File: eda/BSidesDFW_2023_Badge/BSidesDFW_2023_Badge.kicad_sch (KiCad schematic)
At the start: 5 parts

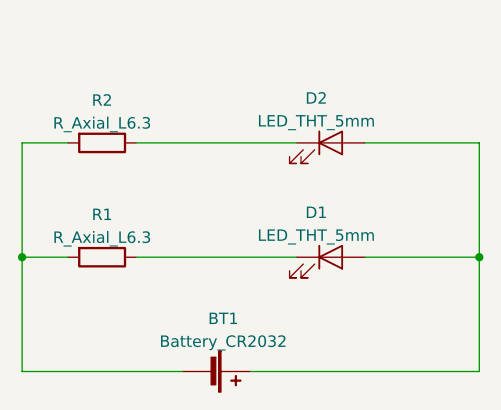
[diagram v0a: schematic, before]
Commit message: document and website updates
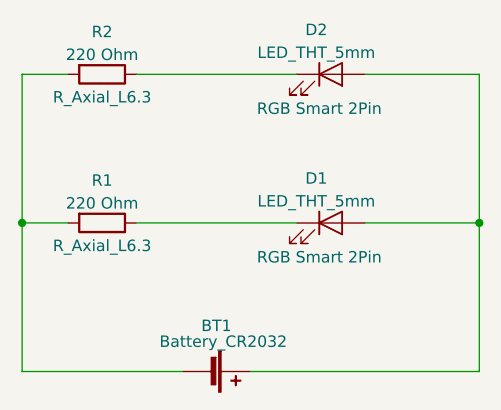
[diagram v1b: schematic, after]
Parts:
- D1, D2: Pkg (none) -> RGB Smart 2Pin
- R1, R2: value R_Axial_L6.3 -> 220 Ohm; Pkg (none) -> R_Axial_L6.3
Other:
- moved on the sheet: D1, D2, R1, R2
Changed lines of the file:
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@@
     (company "Crafted by @alt_bier a.k.a. Richard Gowen")
   )
-  (junction (at 114.3 114.3) (diameter 0) (color 0 0 0 0)
+  (junction (at 165.1 110.49) (diameter 0) (color 0 0 0 0)
   )
-  (junction (at 165.1 114.3) (diameter 0) (color 0 0 0 0)
+  (junction (at 114.3 110.49) (diameter 0) (color 0 0 0 0)
   )
-  (wire (pts (xy 114.3 101.6) (xy 114.3 114.3))
+  (wire (pts (xy 114.3 93.98) (xy 114.3 110.49))
     (stroke (width 0) (type default) (color 0 0 0 0))
   )
-  (wire (pts (xy 165.1 101.6) (xy 152.4 101.6))
+  (wire (pts (xy 165.1 93.98) (xy 152.4 93.98))
     (stroke (width 0) (type default) (color 0 0 0 0))
   )
-  (wire (pts (xy 119.38 101.6) (xy 114.3 101.6))
+  (wire (pts (xy 165.1 110.49) (xy 165.1 93.98))
     (stroke (width 0) (type default) (color 0 0 0 0))
   )
-  (wire (pts (xy 144.78 114.3) (xy 127 114.3))
+  (wire (pts (xy 165.1 110.49) (xy 165.1 127))
     (stroke (width 0) (type default) (color 0 0 0 0))
   )
-  (wire (pts (xy 114.3 114.3) (xy 114.3 127))
+  (wire (pts (xy 119.38 93.98) (xy 114.3 93.98))
+    (stroke (width 0) (type default) (color 0 0 0 0))
+  )
+  (wire (pts (xy 144.78 110.49) (xy 127 110.49))
     (stroke (width 0) (type default) (color 0 0 0 0))
   )
@@
     (stroke (width 0) (type default) (color 0 0 0 0))
   )
-  (wire (pts (xy 144.78 101.6) (xy 127 101.6))
+  (wire (pts (xy 144.78 93.98) (xy 127 93.98))
     (stroke (width 0) (type default) (color 0 0 0 0))
   )
-  (wire (pts (xy 165.1 127) (xy 165.1 114.3))
+  (wire (pts (xy 114.3 110.49) (xy 114.3 127))
     (stroke (width 0) (type default) (color 0 0 0 0))
   )
-  (wire (pts (xy 165.1 114.3) (xy 152.4 114.3))
+  (wire (pts (xy 165.1 110.49) (xy 152.4 110.49))
     (stroke (width 0) (type default) (color 0 0 0 0))
   )
-  (wire (pts (xy 119.38 114.3) (xy 114.3 114.3))
-    (stroke (width 0) (type default) (color 0 0 0 0))
-  )
-  (wire (pts (xy 165.1 114.3) (xy 165.1 101.6))
+  (wire (pts (xy 119.38 110.49) (xy 114.3 110.49))
     (stroke (width 0) (type default) (color 0 0 0 0))
   )
@@
     (stroke (width 0) (type default) (color 0 0 0 0))
   )
-  (symbol (lib_id "0_local:LED_THT_5mm") (at 148.59 114.3 0) (unit 1)
-    (in_bom yes) (on_board yes) (fields_autoplaced)
-    (property "Reference" "D1" (id 0) (at 146.9898 109.3556 0))
-    (property "Value" "LED_THT_5mm" (id 1) (at 146.9898 111.8925 0))
-    (property "Footprint" "0_local:LED_D5.0mm-2" (id 2) (at 148.59 120.65 0)
+  (symbol (lib_id "0_local:LED_THT_5mm") (at 148.59 110.49 0) (unit 1)
+    (in_bom yes) (on_board yes)
+    (property "Reference" "D1" (id 0) (at 146.9898 105.5456 0))
+    (property "Value" "LED_THT_5mm" (id 1) (at 146.9898 108.0825 0))
+    (property "Footprint" "0_local:LED_D5.0mm-2" (id 2) (at 148.59 116.84 0)
       (effects (font (size 1.27 1.27)) hide)
     )
-    (property "Datasheet" "~" (id 3) (at 148.59 114.3 0)
+    (property "Datasheet" "~" (id 3) (at 148.59 110.49 0)
       (effects (font (size 1.27 1.27)) hide)
     )
+    (property "Pkg" "RGB Smart 2Pin" (id 4) (at 147.32 114.3 0))
     (pin "1")
     (pin "2")
   )
-  (symbol (lib_id "0_local:LED_THT_5mm") (at 148.59 101.6 0) (unit 1)
-    (in_bom yes) (on_board yes) (fields_autoplaced)
-    (property "Reference" "D2" (id 0) (at 146.9898 96.6556 0))
-    (property "Value" "LED_THT_5mm" (id 1) (at 146.9898 99.1925 0))
-    (property "Footprint" "0_local:LED_D5.0mm-2" (id 2) (at 148.59 107.95 0)
+  (symbol (lib_id "0_local:LED_THT_5mm") (at 148.59 93.98 0) (unit 1)
+    (in_bom yes) (on_board yes)
+    (property "Reference" "D2" (id 0) (at 146.9898 89.0356 0))
+    (property "Value" "LED_THT_5mm" (id 1) (at 146.9898 91.5725 0))
+    (property "Footprint" "0_local:LED_D5.0mm-2" (id 2) (at 148.59 100.33 0)
       (effects (font (size 1.27 1.27)) hide)
     )
-    (property "Datasheet" "~" (id 3) (at 148.59 101.6 0)
+    (property "Datasheet" "~" (id 3) (at 148.59 93.98 0)
       (effects (font (size 1.27 1.27)) hide)
     )
+    (property "Pkg" "RGB Smart 2Pin" (id 4) (at 147.32 97.79 0))
     (pin "1")
     (pin "2")
   )
-  (symbol (lib_id "0_local:R_Axial_L6.3") (at 123.19 101.6 270) (unit 1)
-    (in_bom yes) (on_board yes) (fields_autoplaced)
-    (property "Reference" "R2" (id 0) (at 123.19 96.8842 90))
-    (property "Value" "R_Axial_L6.3" (id 1) (at 123.19 99.4211 90))
-    (property "Footprint" "0_local:R_Axial_DIN0207_L6.3mm_D2.5mm_P7.62mm_Horizontal_backsilk" (id 2) (at 123.19 97.79 90)
+  (symbol (lib_id "0_local:R_Axial_L6.3") (at 123.19 93.98 270) (unit 1)
+    (in_bom yes) (on_board yes)
+    (property "Reference" "R2" (id 0) (at 123.19 89.2642 90))
+    (property "Value" "220 Ohm" (id 1) (at 123.19 91.8011 90))
+    (property "Footprint" "0_local:R_Axial_DIN0207_L6.3mm_D2.5mm_P7.62mm_Horizontal_backsilk" (id 2) (at 123.19 90.17 90)
       (effects (font (size 1.27 1.27)) hide)
     )
-    (property "Datasheet" "~" (id 3) (at 123.19 99.568 0)
+    (property "Datasheet" "~" (id 3) (at 123.19 91.948 0)
       (effects (font (size 1.27 1.27)) hide)
     )
+    (property "Pkg" " R_Axial_L6.3" (id 4) (at 123.19 96.52 90))
     (pin "1")
     (pin "2")
   )
   (symbol (lib_id "0_local:Battery_CR2032") (at 134.62 127 270) (unit 1)
-    (in_bom yes) (on_board yes) (fields_autoplaced)
-    (property "Reference" "BT1" (id 0) (at 136.652 121.1412 90))
+    (in_bom yes) (on_board yes)
+    (property "Reference" "BT1" (id 0) (at 135.89 121.92 90))
     (property "Value" "Battery_CR2032" (id 1) (at 136.652 123.6781 90))
     (property "Footprint" "0_local:BatteryHolder_CR2032-BS-2-1_Front_backsilk" (id 2) (at 137.414 123.19 90)
@@
     (pin "2")
   )
-  (symbol (lib_id "0_local:R_Axial_L6.3") (at 123.19 114.3 270) (unit 1)
-    (in_bom yes) (on_board yes) (fields_autoplaced)
-    (property "Reference" "R1" (id 0) (at 123.19 109.5842 90))
-    (property "Value" "R_Axial_L6.3" (id 1) (at 123.19 112.1211 90))
-    (property "Footprint" "0_local:R_Axial_DIN0207_L6.3mm_D2.5mm_P7.62mm_Horizontal_backsilk" (id 2) (at 123.19 110.49 90)
+  (symbol (lib_id "0_local:R_Axial_L6.3") (at 123.19 110.49 270) (unit 1)
+    (in_bom yes) (on_board yes)
+    (property "Reference" "R1" (id 0) (at 123.19 105.7742 90))
+    (property "Value" "220 Ohm" (id 1) (at 123.19 108.3111 90))
+    (property "Footprint" "0_local:R_Axial_DIN0207_L6.3mm_D2.5mm_P7.62mm_Horizontal_backsilk" (id 2) (at 123.19 106.68 90)
       (effects (font (size 1.27 1.27)) hide)
     )
-    (property "Datasheet" "~" (id 3) (at 123.19 112.268 0)
+    (property "Datasheet" "~" (id 3) (at 123.19 108.458 0)
       (effects (font (size 1.27 1.27)) hide)
     )
+    (property "Pkg" "R_Axial_L6.3" (id 4) (at 123.19 113.03 90))
     (pin "1")
     (pin "2")
@@
     )
     (path "/f67ac38e-c924-4a3c-ab77-0703b1dd8243"
-      (reference "R1") (unit 1) (value "R_Axial_L6.3") (footprint "0_local:R_Axial_DIN0207_L6.3mm_D2.5mm_P7.62mm_Horizontal_backsilk")
+      (reference "R1") (unit 1) (value "220 Ohm") (footprint "0_local:R_Axial_DIN0207_L6.3mm_D2.5mm_P7.62mm_Horizontal_backsilk")
     )
     (path "/a907f727-cf55-4e58-a189-f5da409b8af3"
-      (reference "R2") (unit 1) (value "R_Axial_L6.3") (footprint "0_local:R_Axial_DIN0207_L6.3mm_D2.5mm_P7.62mm_Horizontal_backsilk")
+      (reference "R2") (unit 1) (value "220 Ohm") (footprint "0_local:R_Axial_DIN0207_L6.3mm_D2.5mm_P7.62mm_Horizontal_backsilk")
     )
   )
